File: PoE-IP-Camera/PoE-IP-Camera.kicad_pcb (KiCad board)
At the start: 4 copper layers, 72.9 x 77.5 mm, 140 parts, among them J1 RJ45, J2 Barrel_Jack_MountingPin, J3 Conn_01x0, J4 Conn_01x04_Socket, J5 Conn_01x04_Socket, P1 USB_C_Plug_USB2.0, SW1 SW_DIP_x03, SW2 434133025816, T1 SM51625EL, U1 TPS54260DGQ, U2 TLP293, U3 CJ431, U5 STM32F030F4Px, Y1 X322525MOB4SI, Y2 X322525MOB4SI

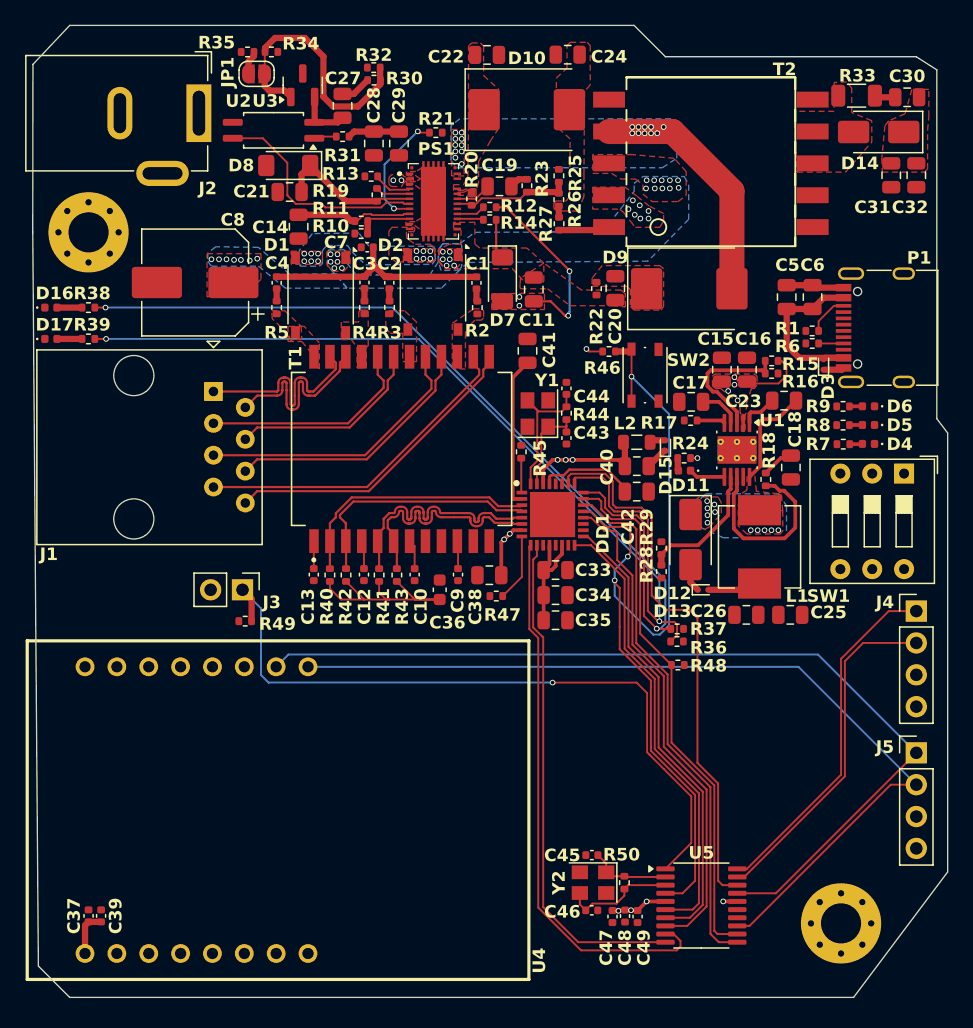
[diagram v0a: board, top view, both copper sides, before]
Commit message: Завершение трассировки
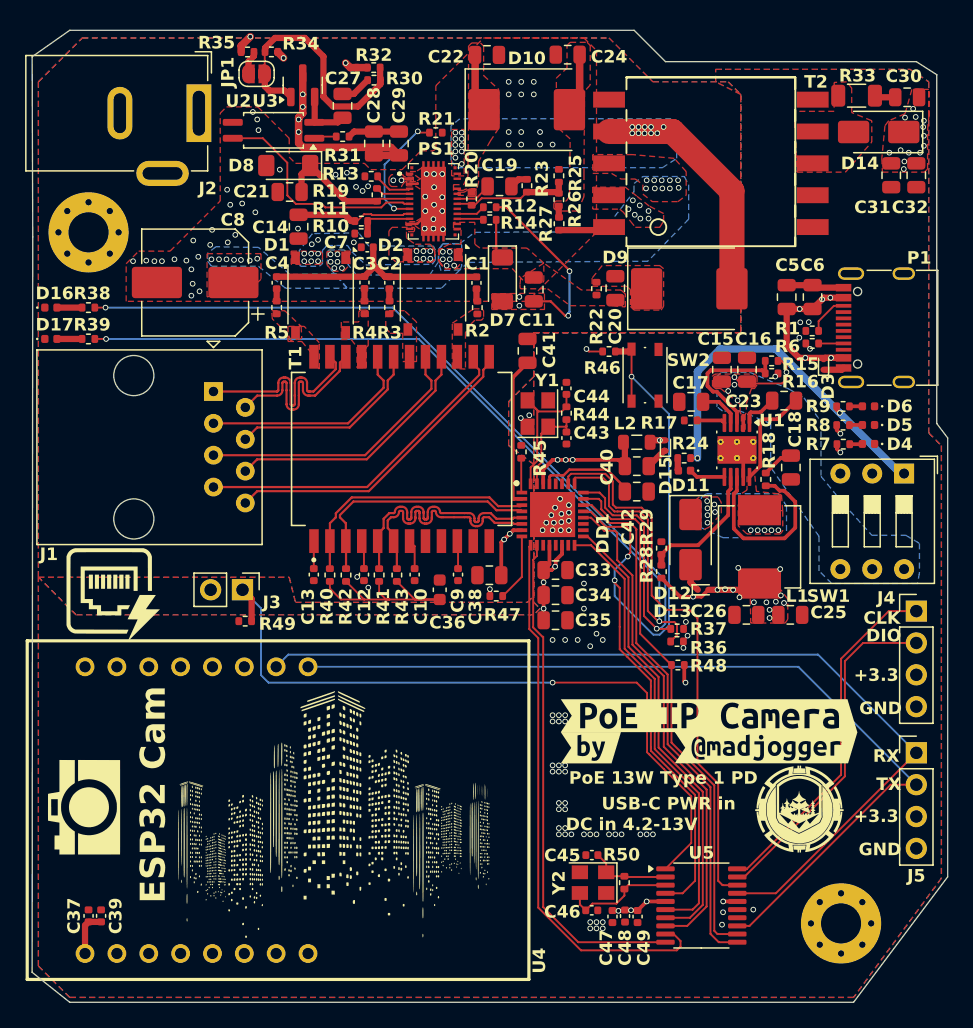
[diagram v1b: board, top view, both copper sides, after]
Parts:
- added G***: LOGO, LOGO, F.Cu at (43.9, 104.7)
- added G***: LOGO, LOGO, B.Cu at (74.5, 58.9)
- added G***: LOGO, LOGO, B.Cu at (59.2, 49.0)
- added G***: LOGO, LOGO, B.Cu at (62.0, 96.4)
- added G***: LOGO, LOGO, B.Cu at (47.4, 53.8)
- added G***: LOGO, LOGO, F.Cu at (23.9, 102.0)
- added G***: LOGO, LOGO, F.Cu at (80.7, 102.5)
- added G***: LOGO, LOGO, F.Cu at (25.8, 85.3)
- added G***: LOGO, LOGO, B.Cu at (26.6, 111.3)
- added G***: LOGO, LOGO, B.Cu at (27.1, 101.3)
- added G***: LOGO, LOGO, B.Cu at (57.4, 70.9)
- added G***: LOGO, LOGO, B.Cu at (68.0, 51.4)
- added G***: LOGO, LOGO, B.Cu at (38.6, 51.3)
- added kibuzzard-67A498E6: G***, kibuzzard-67A498E6, F.Cu at (73.5, 95.0)
- added kibuzzard-67A49B3B: G***, kibuzzard-67A49B3B, F.Cu at (78.0, 97.6)
- added kibuzzard-67A49B47: G***, kibuzzard-67A49B47, F.Cu at (64.0, 97.6)
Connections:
- REF** pad 1: (no net) -> Earth
- U1 pad 11: (no net) -> Earth
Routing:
- net +12V_POE: track 0.55 -> 87.2 mm, vias 1 -> 17
- net +3.3V: track 25.4 -> 68.9 mm, vias 5 -> 26
- net Earth: track 10.4 -> 31.3 mm, vias 0 -> 78
- net Net-(D10-A): track 0.91 -> 5.63 mm
- net Net-(D10-K): track 0.00 -> 4.67 mm
- net GND1: track 0.00 -> 2.72 mm, vias 0 -> 59
- net +5V USB: track 14.4 -> 15.2 mm, vias 0 -> 6
- net Net-(PS1-CP): track 0.00 -> 0.70 mm
- net Net-(U1-VIN): track 6.22 -> 6.39 mm, vias 4 -> 5
- added copper zone on In2.Cu, net +12V_POE
- added copper zone on F.Cu, net +3.3V
- added copper zone on In2.Cu, net +3.3V
- added copper zone on In2.Cu, net +5V USB
- added copper zone on B.Cu, net Earth
- added copper zone on F.Cu, net Earth
- added copper zone on In1.Cu, net Earth
- added copper zone on B.Cu, net Net-(U1-VIN)
- added copper zone on In2.Cu, net VIN
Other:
- board size 72.9 x 77.5 mm -> 73 x 77.5 mm
- board text added: "+3.3"
- board text added: "CLK"
- board text added: "DC in 4.2-13V"
- board text added: "DIO"
- board text added: "ESP32 Cam"
- board text added: "GND"
- board text added: "PoE"
- board text added: "PoE 13W Type 1 PD"
- board text added: "RX"
- board text added: "TX"
- board text added: "USB"
- board text added: "USB-C PWR in"
- board text added: "VIN"
